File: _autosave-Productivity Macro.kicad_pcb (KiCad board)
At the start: 2 copper layers, 34 parts, among them SW1 SW_Push, SW2 Rotary_Encoder_Switch, SW3 Rotary_Encoder_Switch, U1 ATmega32U4-AU, Y1 16Mhz

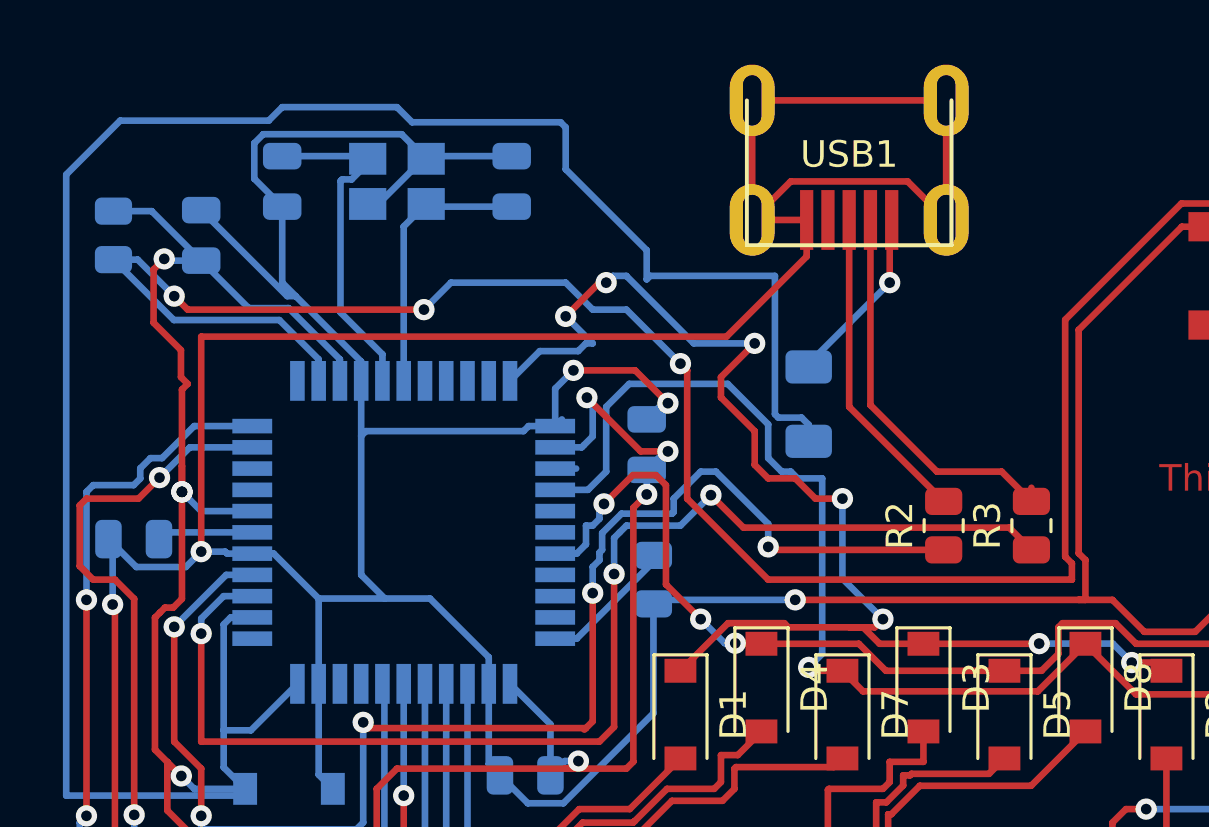
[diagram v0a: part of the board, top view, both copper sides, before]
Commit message: its done
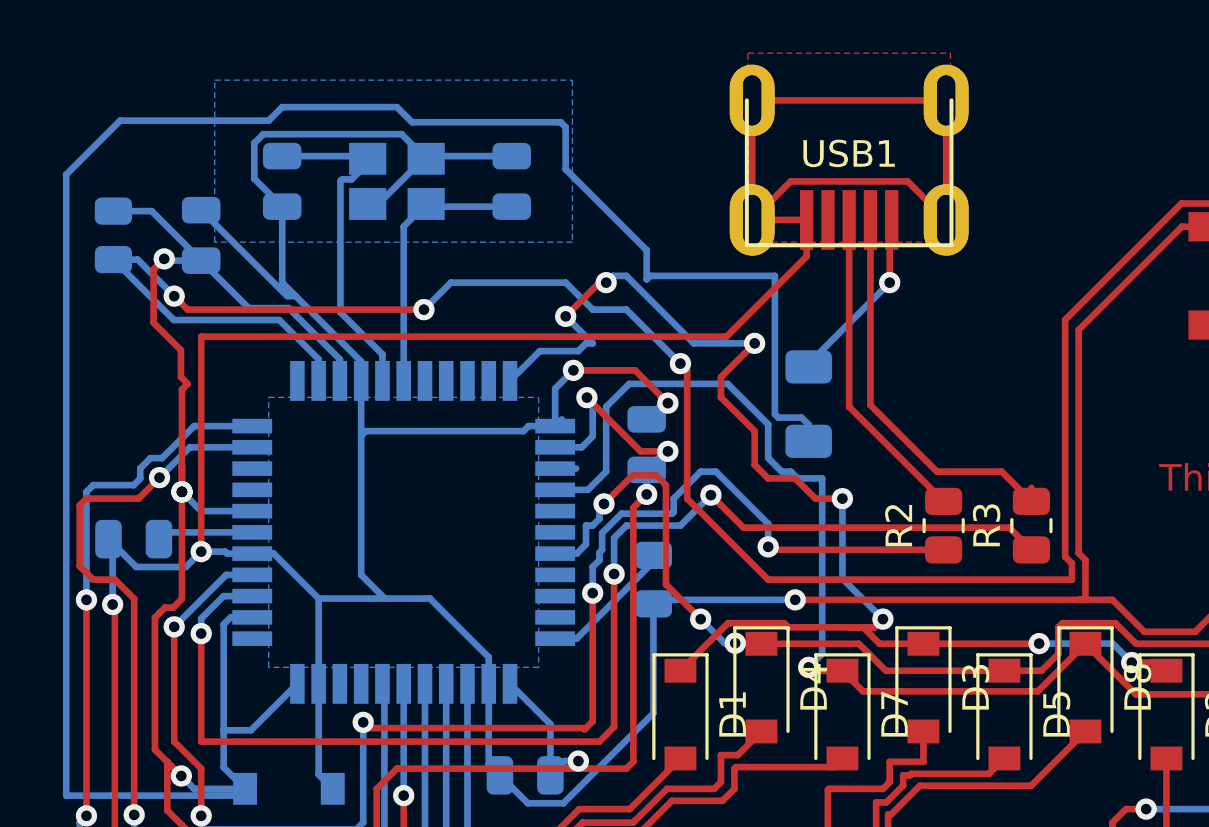
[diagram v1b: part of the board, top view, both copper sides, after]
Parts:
- added G***: LOGO, Logo:Logo, F.Cu at (208.0, 63.2)
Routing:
- added copper zone on B.Cu, net GND
- added copper zone on F.Cu, net GND
